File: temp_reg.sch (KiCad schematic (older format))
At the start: 79 parts

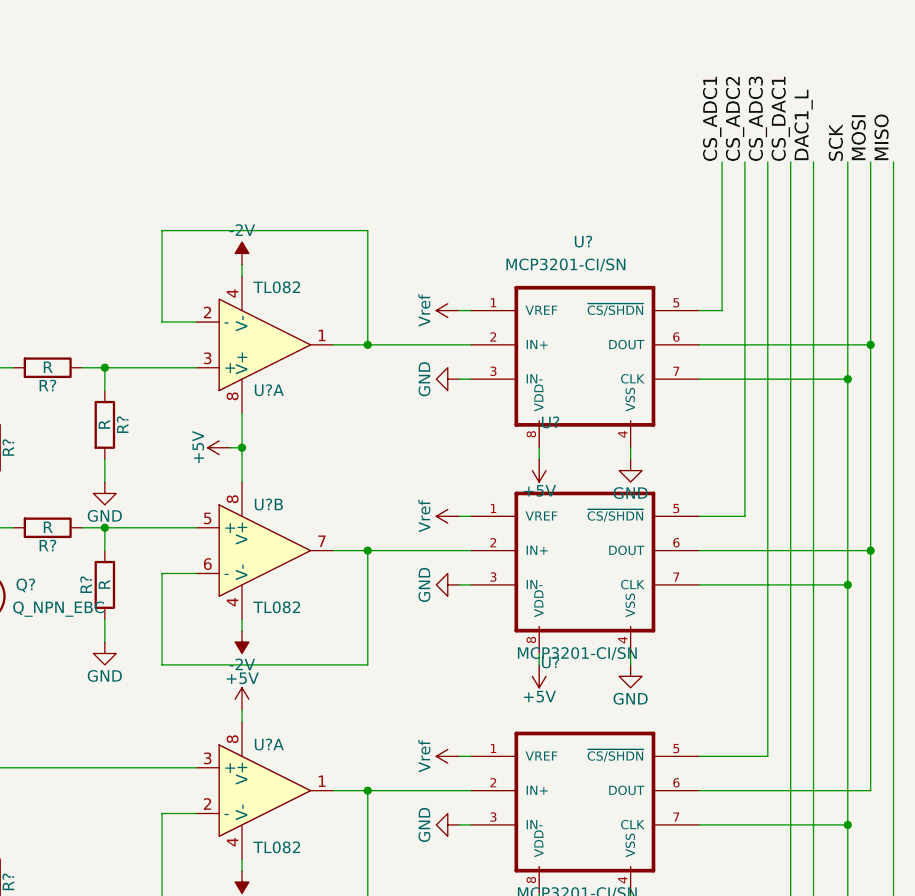
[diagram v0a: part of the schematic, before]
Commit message: initial commit
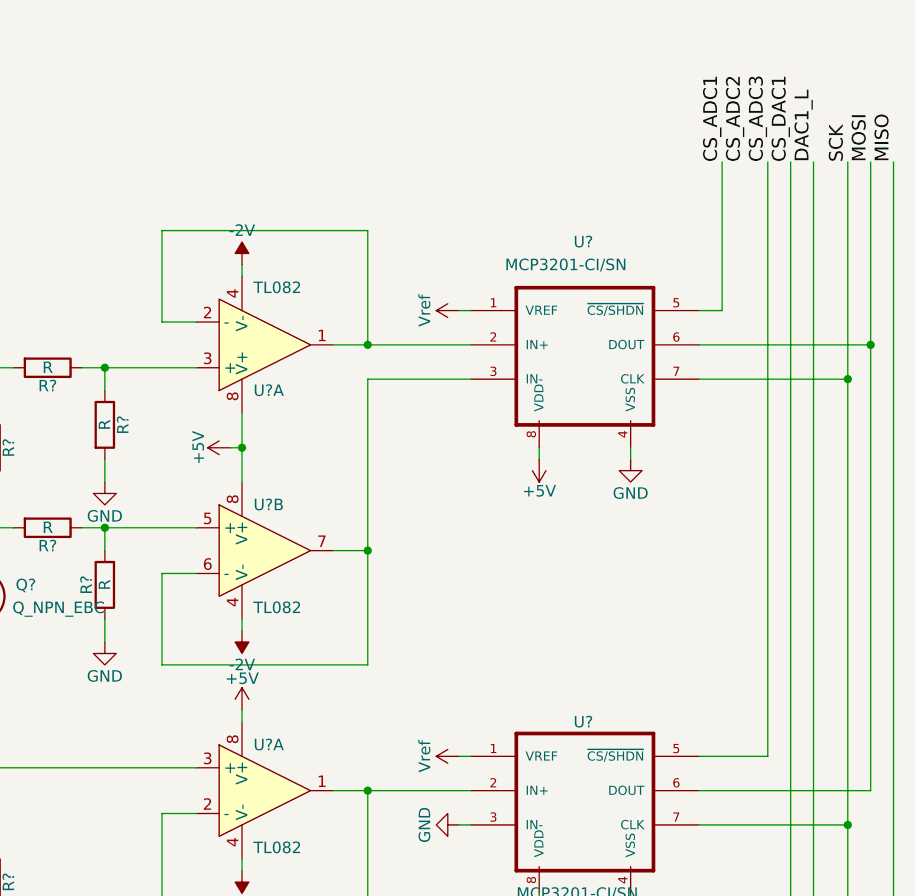
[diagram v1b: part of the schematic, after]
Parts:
- removed U?: MCP3201-CI/SN, SOIC127P600X175-8N, symbol MCP3201-CI/SN-RESCUE-temp_reg-RESCUE-temp_reg
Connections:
- net GND: no longer U?.3 (IN-)
- net at U?.6 (-), U?.7: now also U?.3 (IN-)
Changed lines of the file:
@@
-$Comp
-L MCP3201-CI/SN-RESCUE-temp_reg-RESCUE-temp_reg U?
-U 1 1 57CF970D
-P 18400 4950
-F 0 "U?" H 18206 5559 50  0000 L CNN
-F 1 "MCP3201-CI/SN" H 18100 4550 50  0000 L CNN
-F 2 "SOIC127P600X175-8N" H 18400 4950 50  0001 L CNN
-F 3 "Single Channel SPI Serial Interface 2.7 V 12-Bit A/D Converter SMT - SOIC-8" H 18400 4950 50  0001 L CNN
-F 4 "SOIC-8 Microchip" H 18400 4950 50  0001 L CNN "Package"
-F 5 "Good" H 18400 4950 50  0001 L CNN "Availability"
-F 6 "MCP3201-CI/SN" H 18400 4950 50  0001 L CNN "MP"
-F 7 "2.09 USD" H 18400 4950 50  0001 L CNN "Price"
-F 8 "Microchip" H 18400 4950 50  0001 L CNN "MF"
-	1    18400 4950
-	1    0    0    -1
-$EndComp
 $Comp
 L MCP3201-CI/SN-RESCUE-temp_reg-RESCUE-temp_reg U?
@@
 	16550 5000 16550 5400
 Wire Wire Line
-	16550 5400 17450 5400
-Wire Wire Line
-	17450 5400 17450 4900
-Wire Wire Line
-	17300 4900 17900 4900
+	17450 5400 16550 5400
 Connection ~ 16300 4800
 $Comp
@@
 U 1 1 57D28123
 P 18400 6000
-F 0 "U?" H 18206 6609 50  0000 L CNN
+F 0 "U?" H 18350 6350 50  0000 L CNN
 F 1 "MCP3201-CI/SN" H 18100 5600 50  0000 L CNN
 F 2 "SOIC127P600X175-8N" H 18400 6000 50  0001 L CNN
@@
 $EndComp
 Connection ~ 17450 5950
-Connection ~ 17450 4900
 Wire Wire Line
 	18900 3850 19000 3850
@@
 	19000 3850 19000 3200
 Wire Wire Line
-	18900 4750 19100 4750
-Wire Wire Line
-	19100 4750 19100 3200
-Wire Wire Line
 	18900 5800 19200 5800
 Wire Wire Line
 	17850 3850 17900 3850
-Wire Wire Line
-	17850 4750 17900 4750
 Wire Wire Line
 	17850 5800 17900 5800
@@
 $Comp
 L GND #PWR?
-U 1 1 57D2C9D6
-P 17850 4150
-F 0 "#PWR?" H 17850 3900 50  0001 C CNN
-F 1 "GND" H 17850 4000 50  0000 C CNN
-F 2 "" H 17850 4150 50  0000 C CNN
-F 3 "" H 17850 4150 50  0000 C CNN
-	1    17850 4150
-	0    1    1    0
-$EndComp
-$Comp
-L GND #PWR?
-U 1 1 57D2CC1D
-P 17850 5050
-F 0 "#PWR?" H 17850 4800 50  0001 C CNN
-F 1 "GND" H 17850 4900 50  0000 C CNN
-F 2 "" H 17850 5050 50  0000 C CNN
-F 3 "" H 17850 5050 50  0000 C CNN
-	1    17850 5050
-	0    1    1    0
-$EndComp
-$Comp
-L GND #PWR?
 U 1 1 57D2CE64
 P 17850 6100
@@
 	17850 6100 17900 6100
 Wire Wire Line
-	17850 4150 17900 4150
-Wire Wire Line
-	17850 5050 17900 5050
-$Comp
-L +5V #PWR?
-U 1 1 57D30385
-P 18200 5400
-F 0 "#PWR?" H 18200 5250 50  0001 C CNN
-F 1 "+5V" H 18200 5540 50  0000 C CNN
-F 2 "" H 18200 5400 50  0000 C CNN
-F 3 "" H 18200 5400 50  0000 C CNN
-	1    18200 5400
-	-1   0    0    1
-$EndComp
+	17450 4150 17900 4150
 $Comp
 L +5V #PWR?
@@
 $Comp
 L GND #PWR?
-U 1 1 57D30EFD
-P 18600 5400
-F 0 "#PWR?" H 18600 5150 50  0001 C CNN
-F 1 "GND" H 18600 5250 50  0000 C CNN
-F 2 "" H 18600 5400 50  0000 C CNN
-F 3 "" H 18600 5400 50  0000 C CNN
-	1    18600 5400
-	1    0    0    -1
-$EndComp
-$Comp
-L GND #PWR?
 U 1 1 57D31040
 P 18600 4500
@@
 	1    0    0    -1
 $EndComp
-Wire Wire Line
-	18200 5350 18200 5400
-Wire Wire Line
-	18600 5350 18600 5400
 Wire Wire Line
 	18200 4450 18200 4500
@@
 $Comp
 L Vref #PWR?
-U 1 1 57D8BA27
-P 17850 4750
-F 0 "#PWR?" H 17850 4600 50  0001 C CNN
-F 1 "Vref" H 17850 4900 50  0000 C CNN
-F 2 "" H 17850 4750 50  0000 C CNN
-F 3 "" H 17850 4750 50  0000 C CNN
-	1    17850 4750
-	0    -1   -1   0
-$EndComp
-$Comp
-L Vref #PWR?
 U 1 1 57D8BCB3
 P 17850 5800
@@
 Connection ~ 19550 4150
 Wire Wire Line
-	18900 5050 19550 5050
-Connection ~ 19550 5050
-Wire Wire Line
 	18900 6100 19550 6100
 Connection ~ 19550 6100
@@
 Wire Wire Line
 	19650 4000 18900 4000
-Wire Wire Line
-	19650 4900 18900 4900
 Connection ~ 19650 4000
 Wire Wire Line
 	19650 5950 18900 5950
-Connection ~ 19650 4900
 Wire Wire Line
 	19750 3200 19750 7050
 Wire Wire Line
 	19750 7050 18900 7050
+Wire Wire Line
+	17300 4900 17450 4900
+Wire Wire Line
+	17450 4150 17450 5400
+Connection ~ 17450 4900
 $EndSCHEMATC

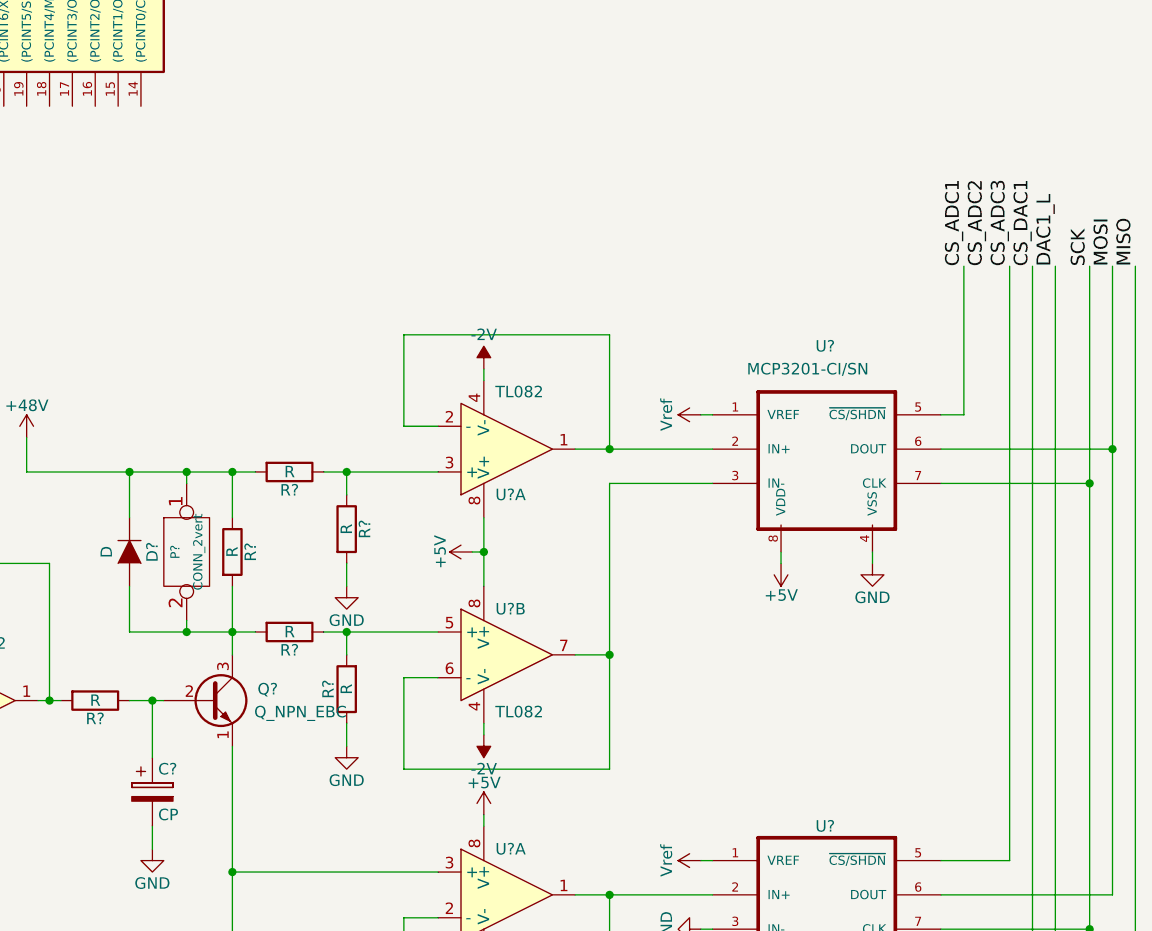
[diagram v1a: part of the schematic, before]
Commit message: 2ADC
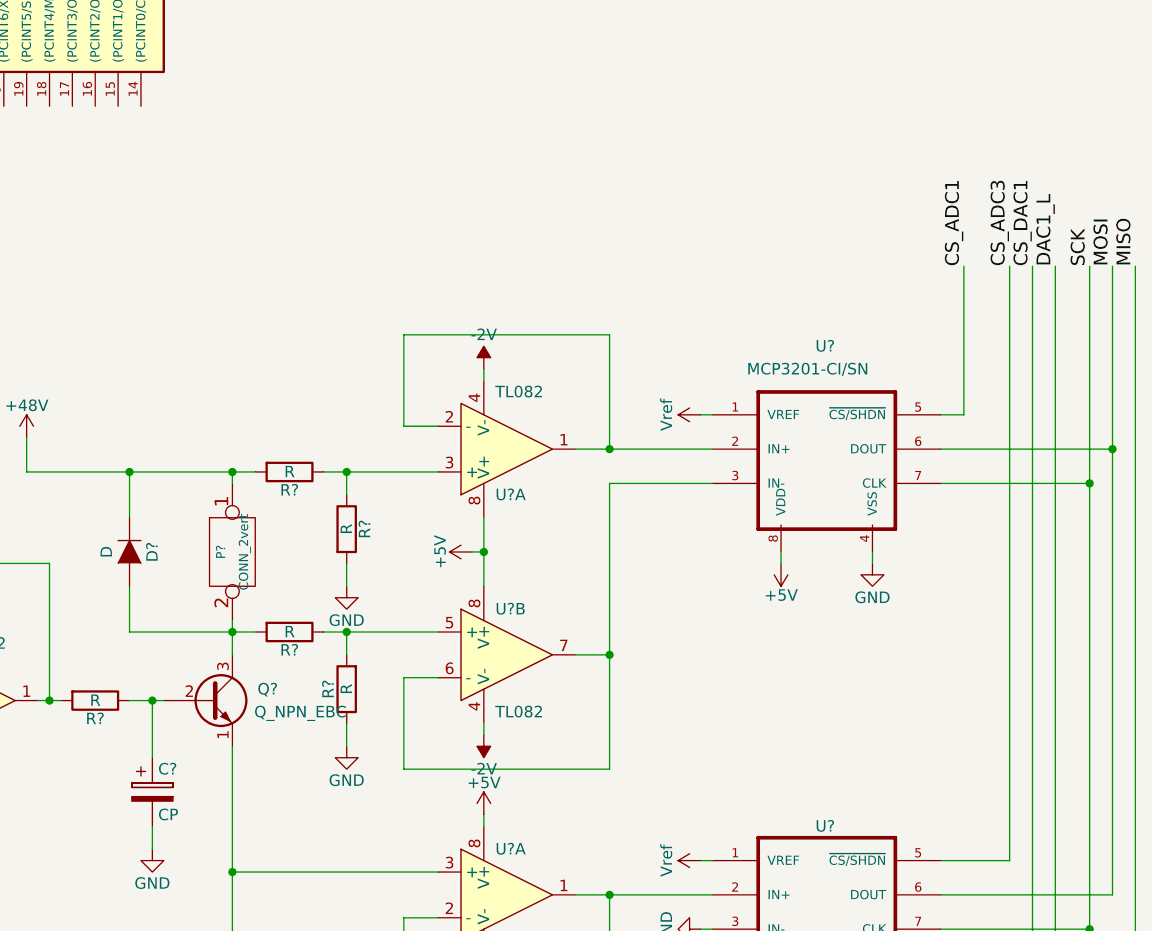
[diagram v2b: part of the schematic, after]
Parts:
- removed R?: R, symbol R
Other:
- moved on the sheet: P?
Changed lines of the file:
@@
-$EndComp
-$Comp
-L R R?
-U 1 1 57CFD088
-P 15800 4450
-F 0 "R?" V 15880 4450 50  0000 C CNN
-F 1 "R" V 15800 4450 50  0000 C CNN
-F 2 "" V 15730 4450 50  0000 C CNN
-F 3 "" H 15800 4450 50  0000 C CNN
-	1    15800 4450
-	1    0    0    -1
 $EndComp
 $Comp
@@
 L CONN_2vert P?
 U 1 1 57D1CC66
-P 15600 4450
-F 0 "P?" V 15550 4450 40  0000 C CNN
-F 1 "CONN_2vert" V 15650 4450 40  0000 C CNN
-F 2 "" H 15600 4450 60  0001 C CNN
-F 3 "" H 15600 4450 60  0001 C CNN
-	1    15600 4450
+P 15800 4450
+F 0 "P?" V 15750 4450 40  0000 C CNN
+F 1 "CONN_2vert" V 15850 4450 40  0000 C CNN
+F 2 "" H 15800 4450 60  0001 C CNN
+F 3 "" H 15800 4450 60  0001 C CNN
+	1    15800 4450
 	1    0    0    -1
 $EndComp
@@
 Connection ~ 2550 7350
 Wire Wire Line
-	15800 4100 15800 4300
-Wire Wire Line
 	14900 4100 15900 4100
 Wire Wire Line
-	15600 4100 15600 4150
-Wire Wire Line
 	14900 4100 14900 3950
-Connection ~ 15600 4100
 Wire Wire Line
 	15350 4600 15350 4800
-Wire Wire Line
-	15350 4800 15900 4800
-Wire Wire Line
-	15800 4600 15800 4900
 Connection ~ 15800 4800
 Wire Wire Line
@@
 Wire Wire Line
 	2850 -1500 2850 -1200
-Wire Wire Line
-	15600 4800 15600 4750
-Connection ~ 15600 4800
 Wire Wire Line
 	15350 4300 15350 4100
@@
 	16550 5000 16550 5400
 Wire Wire Line
-	17450 5400 16550 5400
+	16550 5400 17450 5400
 Connection ~ 16300 4800
 $Comp
@@
 Text Label 19000 3200 1    60   ~ 0
 CS_ADC1
-Text Label 19100 3200 1    60   ~ 0
-CS_ADC2
 Text Label 19200 3200 1    60   ~ 0
 CS_ADC3
@@
 	17300 4900 17450 4900
 Wire Wire Line
-	17450 4150 17450 5400
+	17450 5400 17450 4150
 Connection ~ 17450 4900
+Wire Wire Line
+	15800 4100 15800 4150
+Wire Wire Line
+	15800 4750 15800 4900
+Wire Wire Line
+	15350 4800 15900 4800
 $EndSCHEMATC
